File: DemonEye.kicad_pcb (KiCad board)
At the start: 2 copper layers, 16 x 35.2 mm, 35 parts, among them CN1 PicoBlade 1x07 P1.25mm, Q1 CSD25501F3, Q10 BC807-25QAZ, Q2 CSD25501F3, Q3 CSD25501F3, Q4 CSD25501F3, Q5 CSD25501F3, Q6 BC807-25QAZ, Q8 BC807-25QAZ, Q9 BC807-25QAZ, U1 WS2814F, U2 TLV76701DRVx

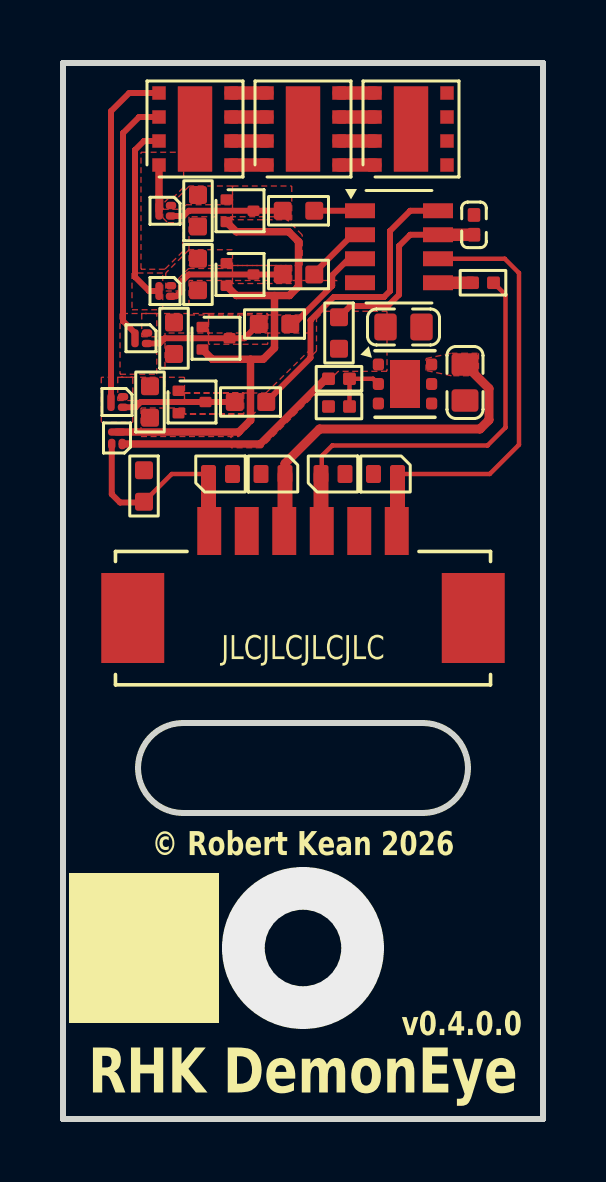
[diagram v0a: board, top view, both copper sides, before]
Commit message: Update ConstantCurrentWithThermalFoldbackDesign.txt, DemonEye.kicad_pcb, DemonEye.kicad_prl, and 3 more files
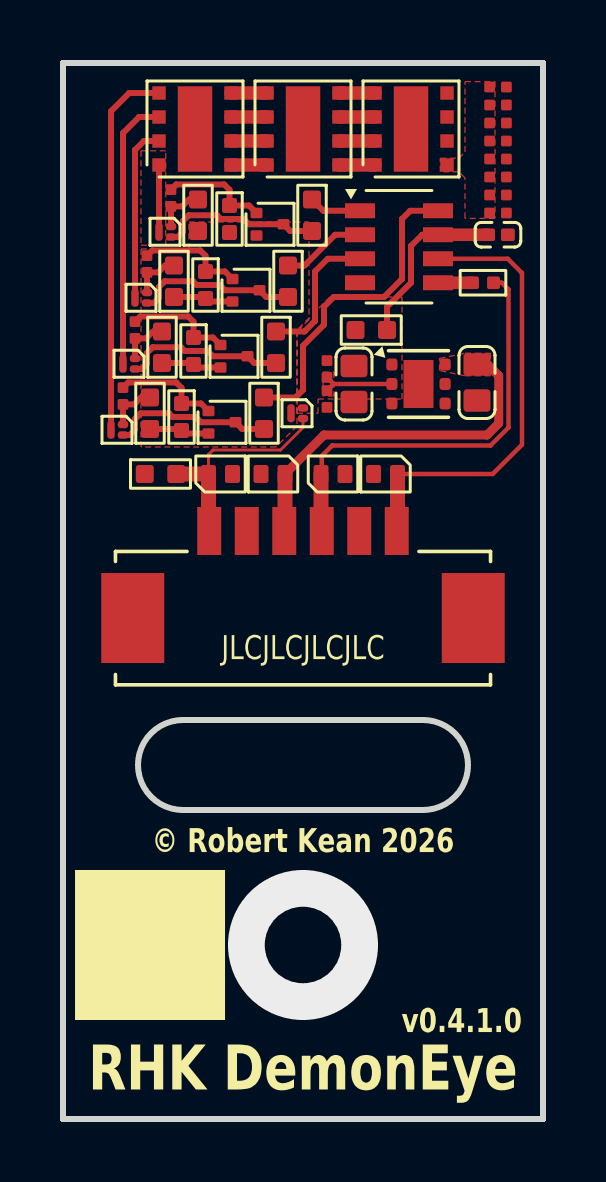
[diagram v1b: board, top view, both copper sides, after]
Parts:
- removed Q10: BC807-25QAZ, My Package_Leadless:DFN1010D-3
- added Q7: BC807-25QAZ, My Package_Leadless:DFN1010D-3, F.Cu at (105.3, 69.2)
- added R14: 1k0, My Resistors:R_0402_Nominal, F.Cu at (106.7, 68.9)
- added R15: 5R6, My Resistors:R_0402_Nominal, F.Cu at (102.5, 71.1)
- added R16: 511, My Resistors:R_0201_Dense, F.Cu at (101.6, 70.5)
- added R17: 1k0, My Resistors:R_0402_Nominal, F.Cu at (106.3, 71.1)
- added R18: 160, My Resistors:R_0201_Dense, F.Cu at (114.1, 60.2)
- added R19: 160, My Resistors:R_0201_Dense, F.Cu at (114.1, 60.8)
- added R20: 160, My Resistors:R_0201_Dense, F.Cu at (114.1, 61.4)
- added R21: 160, My Resistors:R_0201_Dense, F.Cu at (114.1, 62.0)
- added R22: 160, My Resistors:R_0201_Dense, F.Cu at (114.1, 62.6)
- added R23: 160, My Resistors:R_0201_Dense, F.Cu at (114.1, 63.2)
- added R24: 160, My Resistors:R_0201_Dense, F.Cu at (114.1, 63.8)
- added R25: 160, My Resistors:R_0201_Dense, F.Cu at (114.1, 64.4)
- added TH1: 4k7, My Resistors:TH_0402_Nominal, F.Cu at (105.2, 64.6)
- added TH2: 4k7, My Resistors:TH_0402_Nominal, F.Cu at (104.3, 66.8)
- added TH3: 4k7, My Resistors:TH_0402_Nominal, F.Cu at (104.0, 69.0)
- added TH4: 4k7, My Resistors:TH_0402_Nominal, F.Cu at (103.5, 71.2)
- CN1: value PicoBlade 1x07 P1.25mm -> PicoBlade 1x06 P1.25mm
- Q3, Q5: value CSD25501F3 -> BC807-25QAZ; footprint My Package_Leadless:Texas_-YJN_0.7x0.6mm_PicoStar -> My Package_Leadless:DFN1010D-3
- Q6, Q8: value BC807-25QAZ -> CSD25501F3; footprint My Package_Leadless:DFN1010D-3 -> My Package_Leadless:Texas_-YJN_0.7x0.6mm_PicoStar
- R10, R7: value 3R48 -> 511; footprint My Resistors:R_0402_Nominal -> My Resistors:R_0201_Dense
- R11: value 162k -> 1k0; footprint My Resistors:R_0201_Nominal -> My Resistors:R_0402_Nominal
- R12: value 12k7 -> 5R6; footprint My Resistors:R_0201_Nominal -> My Resistors:R_0402_Nominal
- R13: value 33R -> 511; footprint My Resistors:R_0201_Nominal -> My Resistors:R_0201_Dense
- R3: value 1k0 -> 33R; footprint My Resistors:R_0402_Nominal -> My Resistors:R_0201_Nominal
- R4: value 1k0 -> 1M43; footprint My Resistors:R_0402_Nominal -> My Resistors:R_0201_Dense
- R5: value 1k0 -> 105k; footprint My Resistors:R_0402_Nominal -> My Resistors:R_0201_Dense
- R6: value 1k0 -> 5R6
- R8: value 3R48 -> 1k0
- R9: value 3R48 -> 5R6
- moved R13 11.7 mm to (102.0, 68.3), turned to -90 degrees
- moved Q8 6.60 mm to (101.4, 71.6), turned to 180 degrees
- moved R3 6.60 mm to (113.6, 66.7)
- moved R6 6.47 mm to (104.1, 64.5), turned to 90 degrees
- moved Q6 6.30 mm to (101.8, 69.4), turned to 180 degrees
- moved R12 6.22 mm to (102.9, 68.9), turned to 90 degrees
- moved Q1 6.06 mm to (107.4, 71.1), turned to 180 degrees
- moved Q5 5.69 mm to (105.7, 67.0), turned to 0 degrees
- moved R10 4.60 mm to (102.4, 66.1), turned to -90 degrees
- moved R8 4.28 mm to (107.9, 64.5), turned to -90 degrees
- moved Q3 4.15 mm to (106.5, 64.8), turned to 0 degrees
- moved R11 3.67 mm to (107.1, 66.7), turned to -90 degrees
- moved R4 3.29 mm to (108.4, 69.6), turned to 90 degrees
- moved R5 3.05 mm to (108.4, 70.6), turned to 90 degrees
- moved Q9 2.81 mm to (104.9, 71.4)
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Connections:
- LED3 pad 8: GND -> /Red3
- Q2 pad 1: /RedG -> /Gate_{R}
- Q2 pad 2: /RedS -> /Source_{R}
- Q3 pad 1: /GreenG -> /Base_{R}
- Q3 pad 2: /GreenS -> /+V_{OUT_{SW}}
- Q3 pad 3: /Green0 -> /Gate_{R}
- Q4 pad 1: /BlueG -> /Gate_{G}
- Q4 pad 2: /BlueS -> /Source_{G}
- Q4 pad 3: /Blue0 -> /Green0
- Q5 pad 1: /WhiteG -> /Base_{G}
- Q5 pad 2: /WhiteS -> /+V_{OUT_{SW}}
- Q5 pad 3: /White0 -> /Gate_{G}
- Q6 pad 1: /RedS -> /Gate_{B}
- Q6 pad 2: /+V_{OUT_{SW}} -> /Source_{B}
- Q6 pad 3: /RedG -> /Blue0
- Q8 pad 1: /GreenS -> /Gate_{W}
- Q8 pad 2: /+V_{OUT_{SW}} -> /Source_{W}
- Q8 pad 3: /GreenG -> /White0
- Q9 pad 1: /BlueS -> /Base_{W}
- Q9 pad 3: /BlueG -> /Gate_{W}
- R10 pad 1: /+V_{OUT_{SW}} -> /Base_{G}
- R10 pad 2: /WhiteS -> /Source_{G}
- R11 pad 1: /FB -> /OUTG
- R11 pad 2: V_{OUT} -> /Gate_{G}
- R12 pad 1: GND -> /+V_{OUT_{SW}}
- R12 pad 2: /FB -> /Source_{B}
- R13 pad 1: /D_{OUT} -> /Base_{B}
- R13 pad 2: /DOUT -> /Source_{B}
- R3 pad 1: /OUTR -> /D_{OUT}
- R3 pad 2: /RedG -> /DOUT
- R4 pad 1: /OUTG -> /FB
- R4 pad 2: /GreenG -> V_{OUT}
- R5 pad 1: /OUTB -> GND
- R5 pad 2: /BlueG -> /FB
- R6 pad 1: /OUTW -> /+V_{OUT_{SW}}
- R6 pad 2: /WhiteG -> /Source_{R}
- R7 pad 1: /+V_{OUT_{SW}} -> /Base_{R}
- R7 pad 2: /RedS -> /Source_{R}
- R8 pad 1: /+V_{OUT_{SW}} -> /OUTR
- R8 pad 2: /GreenS -> /Gate_{R}
- R9 pad 2: /BlueS -> /Source_{G}
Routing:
- net /+V_{OUT_{SW}}: track 17.9 -> 6.04 mm
- net V_{OUT}: track 7.78 -> 0.00 mm
- net /Gate_{R}: track 0.00 -> 5.43 mm
- net /Gate_{B}: track 0.00 -> 5.43 mm
- net /Gate_{G}: track 0.00 -> 5.43 mm
- net /Gate_{W}: track 0.00 -> 5.43 mm
- net /GreenG: track 4.21 -> 0.00 mm
- net /BlueG: track 3.99 -> 0.00 mm
- net /WhiteG: track 3.80 -> 0.00 mm
- net /RedG: track 3.80 -> 0.00 mm
- net /Base_{R}: track 0.00 -> 3.62 mm
- net /Base_{W}: track 0.00 -> 3.62 mm
- net /Base_{G}: track 0.00 -> 3.62 mm
- net /Base_{B}: track 0.00 -> 3.62 mm
- net /Source_{W}: track 0.00 -> 1.67 mm
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- added copper zone on F.Cu, net /FB
- added copper zone on F.Cu, net /Red3
- removed copper zone on F.Cu, net /Blue0
- removed copper zone on F.Cu, net /BlueG
- removed copper zone on F.Cu, net /BlueS
- removed copper zone on F.Cu, net /Green0
- removed copper zone on F.Cu, net /GreenG
- removed copper zone on F.Cu, net /GreenS
- removed copper zone on F.Cu, net /RedG
- removed copper zone on F.Cu, net /RedS
- removed copper zone on F.Cu, net /White0
- removed copper zone on F.Cu, net /WhiteG
- removed copper zone on F.Cu, net /WhiteS
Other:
- outline, holes or cut-outs redrawn
- board text added: "v0.4.1.0"
- board text removed: "v0.4.0.0"
